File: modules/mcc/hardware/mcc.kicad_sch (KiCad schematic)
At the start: 68 parts, among them J1 PJ301M-12, J11 PJ301M-12, J12 PJ301M-12, J13 PJ301M-12, J14 PJ301M-12, J2 PJ301M-12, J3 Eurorack_2x5, J4 UPDI, Q1 MMBT3904, SW1 BANK, U1 ATtiny1616-MNR, U2 HT7550-1, U3 CJ431, U4 MCP6002, U5 MCP6002

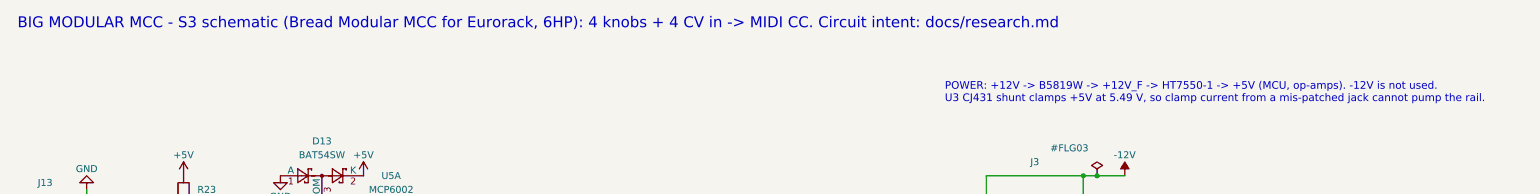
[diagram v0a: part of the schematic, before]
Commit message: Improve MCC.
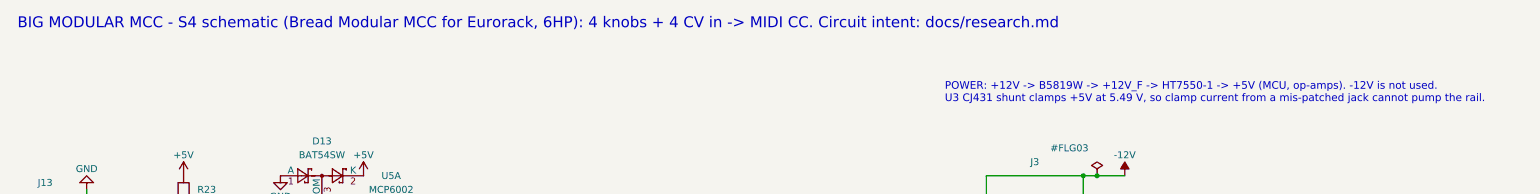
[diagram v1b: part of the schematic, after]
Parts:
- R4: footprint MCC:R_0805_2012Metric -> MCC:R_1206_3216Metric; LCSC C17513 -> C2074262; MPN 0805W8F1001T5E -> ESR18EZPF1001; Manufacturer UNI-ROYAL -> ROHM Semicon; Note Output series 1k (0805, as MIDI V2): <= 6.7 mA / 45 mW into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 -> Output series 1k, 0.5 W 1206 (as 8bit R12): a permanent -12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; Power (none) -> 0.5W
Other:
- note added: "BIG MODULAR MCC - S4 schematic (Bread Modular MCC for Eurorack, 6HP): 4 knobs + 4 CV in -> MIDI CC. Circuit intent: docs/research.md"
- note removed: "BIG MODULAR MCC - S3 schematic (Bread Modular MCC for Eurorack, 6HP): 4 knobs + 4 CV in -> MIDI CC. Circuit intent: docs/research.md"
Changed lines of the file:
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@@
 	(title_block
 		(title "Big Modular - MCC")
-		(rev "S3")
+		(rev "S4")
 		(company "Big Modular")
-		(comment 1 "SCHEMATIC S3 - BM MCC for Eurorack: 4 knobs + 4 CV in -> MIDI CC")
+		(comment 1 "SCHEMATIC S4 - BM MCC for Eurorack: 4 knobs + 4 CV in -> MIDI CC")
 		(comment 2 "Circuit intent: docs/research.md; placement: docs/geometry.json")
 	)
@@
 		)
 	)
-	(text "BIG MODULAR MCC - S3 schematic (Bread Modular MCC for Eurorack, 6HP): 4 knobs + 4 CV in -> MIDI CC. Circuit intent: docs/research.md"
+	(text "BIG MODULAR MCC - S4 schematic (Bread Modular MCC for Eurorack, 6HP): 4 knobs + 4 CV in -> MIDI CC. Circuit intent: docs/research.md"
 		(exclude_from_sim no)
 		(at 20.32 17.78 0)
@@
 			)
 		)
-		(property "Footprint" "MCC:R_0805_2012Metric"
+		(property "Footprint" "MCC:R_1206_3216Metric"
 			(at 226.06 254 90)
 			(hide yes)
@@
 			)
 		)
-		(property "Note" "Output series 1k (0805, as MIDI V2): <= 6.7 mA / 45 mW into the clamp on a +/-12 V mis-patch"
+		(property "Power" "0.5W"
 			(at 226.06 254 90)
 			(hide yes)
@@
 			)
 		)
-		(property "LCSC" "C17513"
+		(property "Note" "Output series 1k, 0.5 W 1206 (as 8bit R12): a permanent -12 V on the tip against PB2 idling high is ~17 V / 0.29 W (+12 V into the +5V clamp: 45 mW)"
 			(at 226.06 254 90)
 			(hide yes)
@@
 			)
 		)
-		(property "MPN" "0805W8F1001T5E"
+		(property "LCSC" "C2074262"
 			(at 226.06 254 90)
 			(hide yes)
@@
 			)
 		)
-		(property "Manufacturer" "UNI-ROYAL"
+		(property "MPN" "ESR18EZPF1001"
+			(at 226.06 254 90)
+			(hide yes)
+			(show_name no)
+			(do_not_autoplace no)
+			(effects
+				(font
+					(size 1.27 1.27)
+				)
+			)
+		)
+		(property "Manufacturer" "ROHM Semicon"
 			(at 226.06 254 90)
 			(hide yes)
